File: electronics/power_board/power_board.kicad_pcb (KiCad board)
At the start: 2 copper layers, 44.5 x 39.4 mm, 38 parts, among them J1 Vin, J4 3.3V out, J5 5V out, J7 Vin, U1 TPS54228, U2 TPS54228

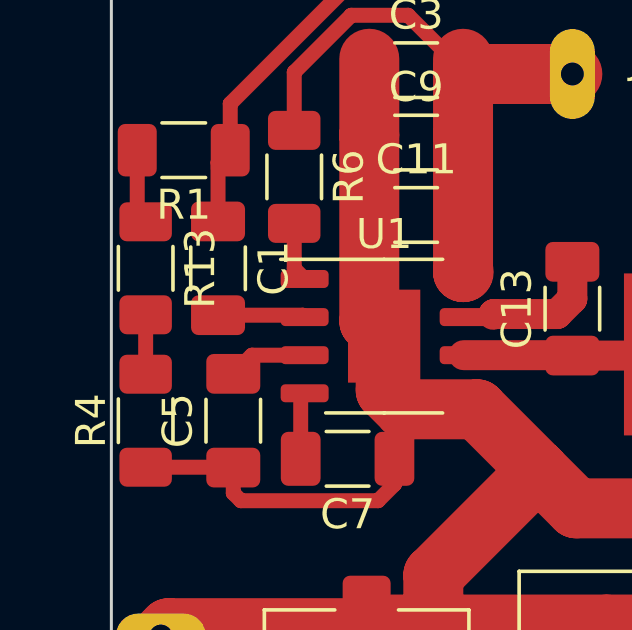
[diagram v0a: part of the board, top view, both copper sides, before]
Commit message: 3d renders of electronics
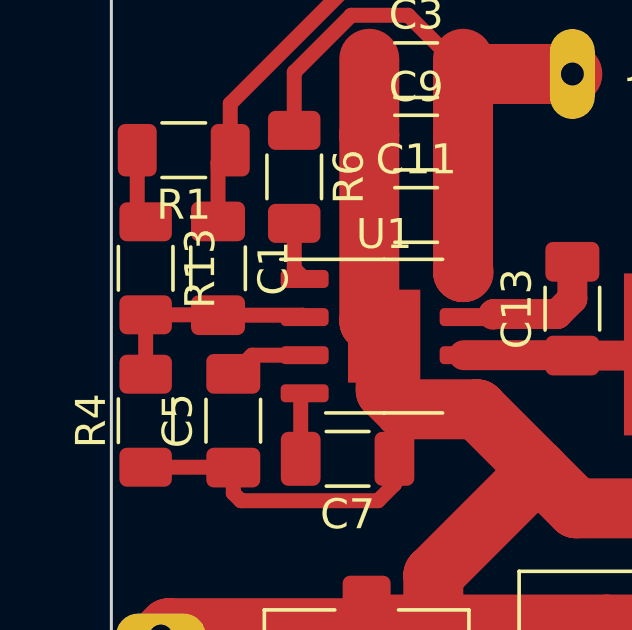
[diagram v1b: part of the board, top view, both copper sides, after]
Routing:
- net Net-(C1-Pad2): track 4.89 -> 7.31 mm
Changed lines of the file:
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@@
+      (rotate (xyz 0 0 0))
+    )
+    (model "${KICAD6_3DMODEL_DIR}/Inductor_SMD.3dshapes/L_TDK_SLF12575.wrl"
+      (offset (xyz 0 0 0))
+      (scale (xyz 1 1 1))
       (rotate (xyz 0 0 0))
     )
@@
       (rotate (xyz 0 0 0))
     )
+    (model "${KICAD6_3DMODEL_DIR}/Inductor_SMD.3dshapes/L_TDK_SLF12575.wrl"
+      (offset (xyz 0 0 0))
+      (scale (xyz 1 1 1))
+      (rotate (xyz 0 0 0))
+    )
   )
   (footprint "moje:ARK" (layer "F.Cu")
@@
   (segment (start 123.3471 33.4395) (end 123.4102 33.5026) (width 0.5) (layer "F.Cu") (net 2))
   (segment (start 120.523 33.4395) (end 123.3471 33.4395) (width 0.5) (layer "F.Cu") (net 2))
+  (segment (start 118.11 33.427) (end 120.5105 33.427) (width 0.5) (layer "F.Cu") (net 2))
+  (segment (start 120.5105 33.427) (end 120.523 33.4395) (width 0.5) (layer "F.Cu") (net 2))
   (segment (start 118.11 35.407) (end 118.11 33.427) (width 0.5) (layer "F.Cu") (net 2))
   (segment (start 120.009 55.245) (end 120.009 50.6035) (width 2) (layer "F.Cu") (net 3))
